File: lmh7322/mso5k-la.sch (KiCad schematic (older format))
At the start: 4 parts, among them J1 output, J2 input

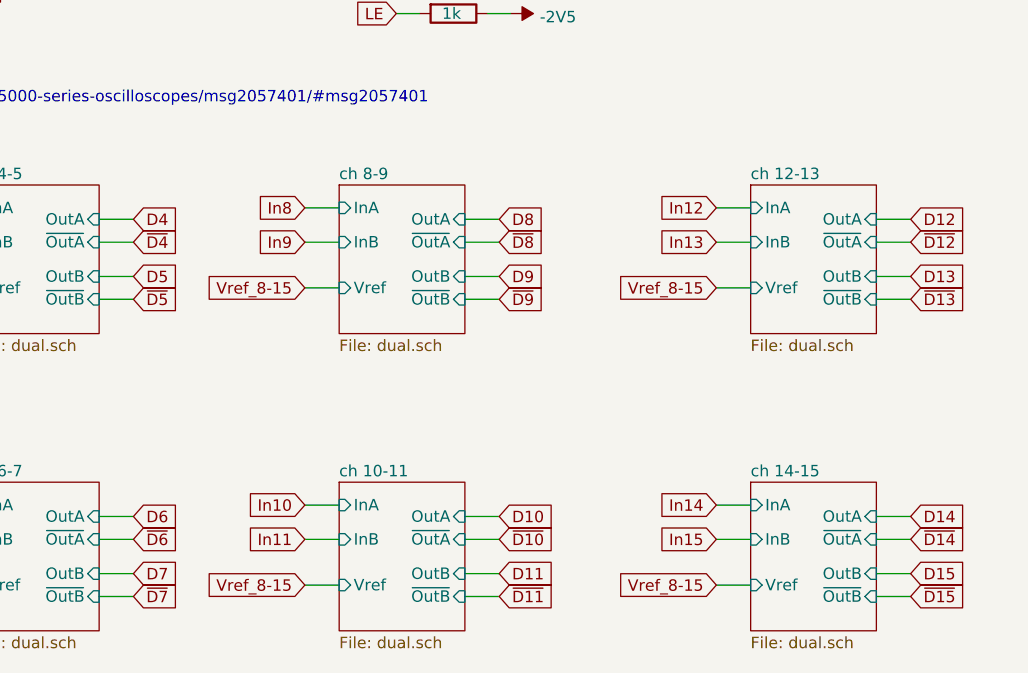
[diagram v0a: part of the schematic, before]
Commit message: Minor cleanup
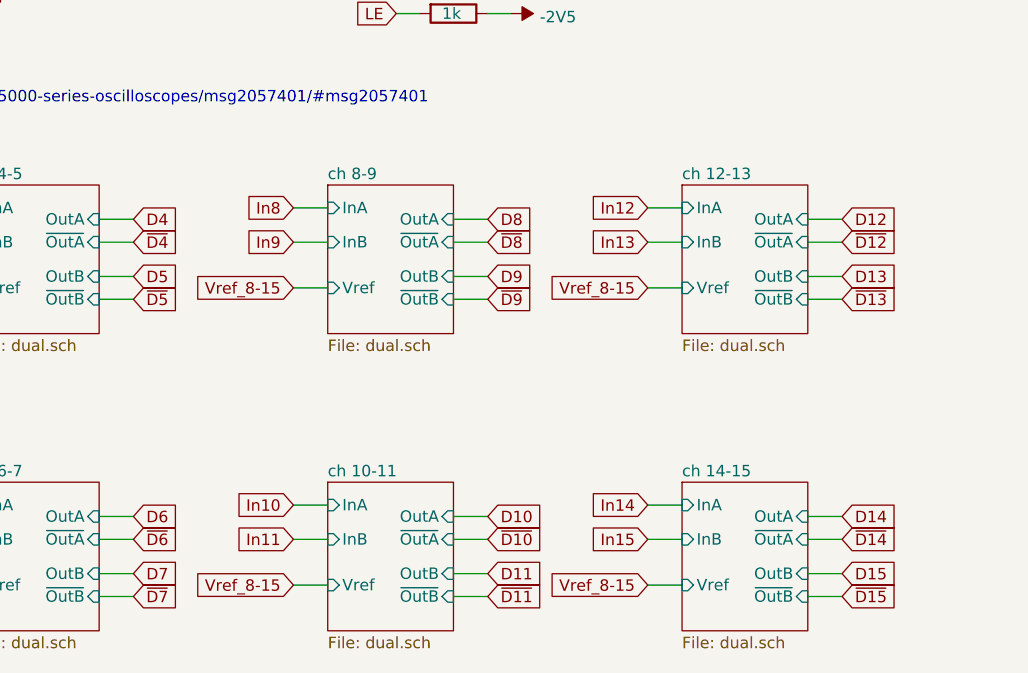
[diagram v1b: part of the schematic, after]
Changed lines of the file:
@@
 Wire Wire Line
 	3650 4450 3800 4450
-Text GLabel 4550 4400 0    50   Input ~ 0
+Text GLabel 4500 4400 0    50   Input ~ 0
 In8
-Text GLabel 4550 4550 0    50   Input ~ 0
+Text GLabel 4500 4550 0    50   Input ~ 0
 In9
 Wire Wire Line
-	4550 4400 4700 4400
-Wire Wire Line
-	4550 4550 4700 4550
-Text GLabel 4550 5700 0    50   Input ~ 0
+	4500 4400 4650 4400
+Wire Wire Line
+	4500 4550 4650 4550
+Text GLabel 4500 5700 0    50   Input ~ 0
 In10
-Text GLabel 4550 5850 0    50   Input ~ 0
+Text GLabel 4500 5850 0    50   Input ~ 0
 In11
 Wire Wire Line
-	4700 5700 4550 5700
-Wire Wire Line
-	4700 5850 4550 5850
-Text GLabel 5400 4700 2    50   Input ~ 0
+	4650 5700 4500 5700
+Wire Wire Line
+	4650 5850 4500 5850
+Text GLabel 5350 4700 2    50   Input ~ 0
 D9
-Text GLabel 5400 4800 2    50   Input ~ 0
+Text GLabel 5350 4800 2    50   Input ~ 0
 ~D9
-Text GLabel 5400 4450 2    50   Input ~ 0
+Text GLabel 5350 4450 2    50   Input ~ 0
 D8
-Text GLabel 5400 4550 2    50   Input ~ 0
+Text GLabel 5350 4550 2    50   Input ~ 0
 ~D8
-Text GLabel 5400 6000 2    50   Input ~ 0
+Text GLabel 5350 6000 2    50   Input ~ 0
 D11
-Text GLabel 5400 6100 2    50   Input ~ 0
+Text GLabel 5350 6100 2    50   Input ~ 0
 ~D11
-Text GLabel 5400 5750 2    50   Input ~ 0
+Text GLabel 5350 5750 2    50   Input ~ 0
 D10
-Text GLabel 5400 5850 2    50   Input ~ 0
+Text GLabel 5350 5850 2    50   Input ~ 0
 ~D10
 Wire Wire Line
-	5400 6100 5250 6100
-Wire Wire Line
-	5250 6000 5400 6000
-Wire Wire Line
-	5400 5850 5250 5850
-Wire Wire Line
-	5250 5750 5400 5750
-Wire Wire Line
-	5400 4800 5250 4800
-Wire Wire Line
-	5250 4700 5400 4700
-Wire Wire Line
-	5400 4550 5250 4550
-Wire Wire Line
-	5250 4450 5400 4450
-Text GLabel 6350 4400 0    50   Input ~ 0
+	5350 6100 5200 6100
+Wire Wire Line
+	5200 6000 5350 6000
+Wire Wire Line
+	5350 5850 5200 5850
+Wire Wire Line
+	5200 5750 5350 5750
+Wire Wire Line
+	5350 4800 5200 4800
+Wire Wire Line
+	5200 4700 5350 4700
+Wire Wire Line
+	5350 4550 5200 4550
+Wire Wire Line
+	5200 4450 5350 4450
+Text GLabel 6050 4400 0    50   Input ~ 0
 In12
-Text GLabel 6350 4550 0    50   Input ~ 0
+Text GLabel 6050 4550 0    50   Input ~ 0
 In13
 Wire Wire Line
-	6350 4400 6500 4400
-Wire Wire Line
-	6350 4550 6500 4550
-Text GLabel 6350 5700 0    50   Input ~ 0
+	6050 4400 6200 4400
+Wire Wire Line
+	6050 4550 6200 4550
+Text GLabel 6050 5700 0    50   Input ~ 0
 In14
-Text GLabel 6350 5850 0    50   Input ~ 0
+Text GLabel 6050 5850 0    50   Input ~ 0
 In15
 Wire Wire Line
-	6500 5700 6350 5700
-Wire Wire Line
-	6500 5850 6350 5850
-Text GLabel 7200 4700 2    50   Input ~ 0
+	6200 5700 6050 5700
+Wire Wire Line
+	6200 5850 6050 5850
+Text GLabel 6900 4700 2    50   Input ~ 0
 D13
-Text GLabel 7200 4800 2    50   Input ~ 0
+Text GLabel 6900 4800 2    50   Input ~ 0
 ~D13
-Text GLabel 7200 4450 2    50   Input ~ 0
+Text GLabel 6900 4450 2    50   Input ~ 0
 D12
-Text GLabel 7200 4550 2    50   Input ~ 0
+Text GLabel 6900 4550 2    50   Input ~ 0
 ~D12
-Text GLabel 7200 6000 2    50   Input ~ 0
+Text GLabel 6900 6000 2    50   Input ~ 0
 D15
-Text GLabel 7200 6100 2    50   Input ~ 0
+Text GLabel 6900 6100 2    50   Input ~ 0
 ~D15
-Text GLabel 7200 5750 2    50   Input ~ 0
+Text GLabel 6900 5750 2    50   Input ~ 0
 D14
-Text GLabel 7200 5850 2    50   Input ~ 0
+Text GLabel 6900 5850 2    50   Input ~ 0
 ~D14
 Wire Wire Line
-	7200 6100 7050 6100
-Wire Wire Line
-	7050 6000 7200 6000
-Wire Wire Line
-	7200 5850 7050 5850
-Wire Wire Line
-	7050 5750 7200 5750
-Wire Wire Line
-	7200 4800 7050 4800
-Wire Wire Line
-	7050 4700 7200 4700
-Wire Wire Line
-	7200 4550 7050 4550
-Wire Wire Line
-	7050 4450 7200 4450
+	6900 6100 6750 6100
+Wire Wire Line
+	6750 6000 6900 6000
+Wire Wire Line
+	6900 5850 6750 5850
+Wire Wire Line
+	6750 5750 6900 5750
+Wire Wire Line
+	6900 4800 6750 4800
+Wire Wire Line
+	6750 4700 6900 4700
+Wire Wire Line
+	6900 4550 6750 4550
+Wire Wire Line
+	6750 4450 6900 4450
 Text GLabel 1450 6050 0    50   Input ~ 0
 Vref_0-7
@@
 Wire Wire Line
 	3100 6050 2950 6050
-Text GLabel 4550 6050 0    50   Input ~ 0
+Text GLabel 4500 6050 0    50   Input ~ 0
 Vref_8-15
-Text GLabel 6350 6050 0    50   Input ~ 0
+Text GLabel 6050 6050 0    50   Input ~ 0
 Vref_8-15
 Wire Wire Line
-	6350 6050 6500 6050
-Wire Wire Line
-	4700 6050 4550 6050
+	6050 6050 6200 6050
+Wire Wire Line
+	4650 6050 4500 6050
 Text Notes 1050 3950 0    50   ~ 0
 For reference see:\nhttp://www.eevblog.com/forum/testgear/hacking-the-rigol-mso5000-series-oscilloscopes/msg2057401/#msg2057401
@@
 $EndSheet
 $Sheet
-S 4700 5600 550  650
+S 4650 5600 550  650
 U 5C4E2524
 F0 "ch 10-11" 50
 F1 "dual.sch" 50
-F2 "InB" I L 4700 5850 50
-F3 "Vref" I L 4700 6050 50
-F4 "OutA" I R 5250 5750 50
-F5 "~OutA" I R 5250 5850 50
-F6 "InA" I L 4700 5700 50
-F7 "OutB" I R 5250 6000 50
-F8 "~OutB" I R 5250 6100 50
-$EndSheet
-$Sheet
-S 4700 4300 550  650
+F2 "InB" I L 4650 5850 50
+F3 "Vref" I L 4650 6050 50
+F4 "OutA" I R 5200 5750 50
+F5 "~OutA" I R 5200 5850 50
+F6 "InA" I L 4650 5700 50
+F7 "OutB" I R 5200 6000 50
+F8 "~OutB" I R 5200 6100 50
+$EndSheet
+$Sheet
+S 4650 4300 550  650
 U 5C4E98BE
 F0 "ch 8-9" 50
 F1 "dual.sch" 50
-F2 "InB" I L 4700 4550 50
-F3 "Vref" I L 4700 4750 50
-F4 "OutA" I R 5250 4450 50
-F5 "~OutA" I R 5250 4550 50
-F6 "InA" I L 4700 4400 50
-F7 "OutB" I R 5250 4700 50
-F8 "~OutB" I R 5250 4800 50
-$EndSheet
-$Sheet
-S 6500 4300 550  650
+F2 "InB" I L 4650 4550 50
+F3 "Vref" I L 4650 4750 50
+F4 "OutA" I R 5200 4450 50
+F5 "~OutA" I R 5200 4550 50
+F6 "InA" I L 4650 4400 50
+F7 "OutB" I R 5200 4700 50
+F8 "~OutB" I R 5200 4800 50
+$EndSheet
+$Sheet
+S 6200 4300 550  650
 U 5C4E98C7
 F0 "ch 12-13" 50
 F1 "dual.sch" 50
-F2 "InB" I L 6500 4550 50
-F3 "Vref" I L 6500 4750 50
-F4 "OutA" I R 7050 4450 50
-F5 "~OutA" I R 7050 4550 50
-F6 "InA" I L 6500 4400 50
-F7 "OutB" I R 7050 4700 50
-F8 "~OutB" I R 7050 4800 50
-$EndSheet
-$Sheet
-S 6500 5600 550  650
+F2 "InB" I L 6200 4550 50
+F3 "Vref" I L 6200 4750 50
+F4 "OutA" I R 6750 4450 50
+F5 "~OutA" I R 6750 4550 50
+F6 "InA" I L 6200 4400 50
+F7 "OutB" I R 6750 4700 50
+F8 "~OutB" I R 6750 4800 50
+$EndSheet
+$Sheet
+S 6200 5600 550  650
 U 5C4E98D0
 F0 "ch 14-15" 50
 F1 "dual.sch" 50
-F2 "InB" I L 6500 5850 50
-F3 "Vref" I L 6500 6050 50
-F4 "OutA" I R 7050 5750 50
-F5 "~OutA" I R 7050 5850 50
-F6 "InA" I L 6500 5700 50
-F7 "OutB" I R 7050 6000 50
-F8 "~OutB" I R 7050 6100 50
+F2 "InB" I L 6200 5850 50
+F3 "Vref" I L 6200 6050 50
+F4 "OutA" I R 6750 5750 50
+F5 "~OutA" I R 6750 5850 50
+F6 "InA" I L 6200 5700 50
+F7 "OutB" I R 6750 6000 50
+F8 "~OutB" I R 6750 6100 50
 $EndSheet
 Text GLabel 2950 4750 0    50   Input ~ 0
@@
 Wire Wire Line
 	2950 4750 3100 4750
-Text GLabel 4550 4750 0    50   Input ~ 0
+Text GLabel 4500 4750 0    50   Input ~ 0
 Vref_8-15
 Wire Wire Line
-	4550 4750 4700 4750
-Text GLabel 6350 4750 0    50   Input ~ 0
+	4500 4750 4650 4750
+Text GLabel 6050 4750 0    50   Input ~ 0
 Vref_8-15
 Wire Wire Line
-	6350 4750 6500 4750
+	6050 4750 6200 4750
 $EndSCHEMATC
